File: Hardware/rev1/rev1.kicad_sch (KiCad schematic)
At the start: 0 parts

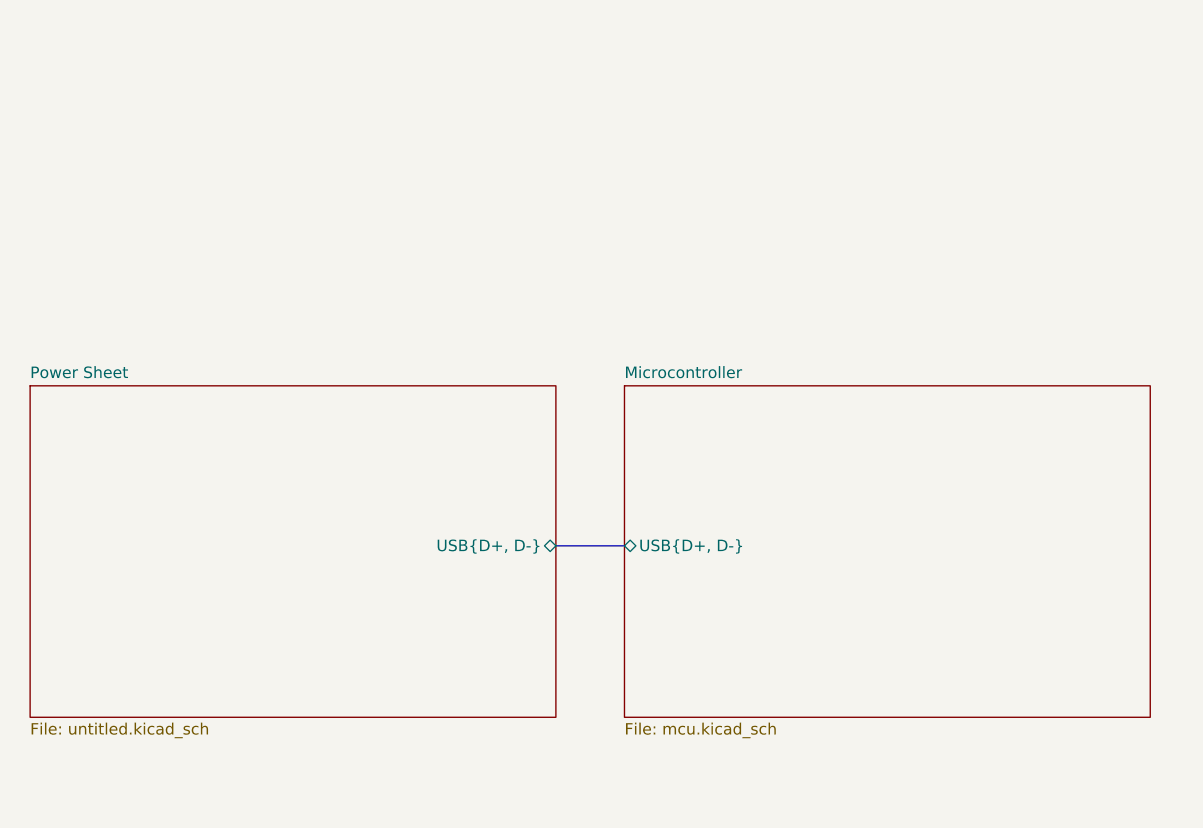
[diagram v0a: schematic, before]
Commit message: Add buses (maybe)
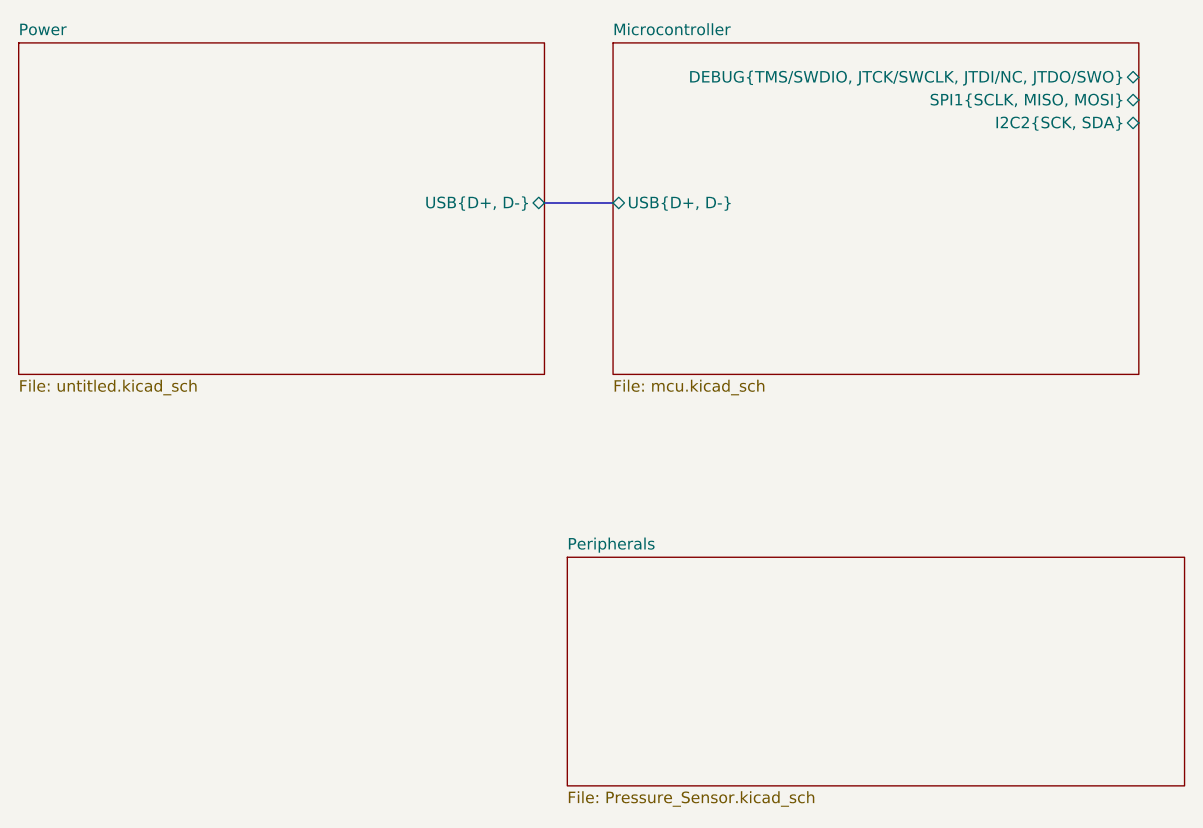
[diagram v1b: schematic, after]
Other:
- sheet Power Sheet renamed Power
- added sheet Peripherals (Pressure_Sensor.kicad_sch)
- sheet Microcontroller ports: added DEBUG{TMS/SWDIO, JTCK/SWCLK, JTDI/NC, JTDO/SWO}, I2C2{SCK, SDA}, SPI1{SCLK, MISO, MOSI}; removed none
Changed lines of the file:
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@@
 	(bus
 		(pts
-			(xy 144.78 95.25) (xy 152.4 95.25)
+			(xy 143.51 57.15) (xy 151.13 57.15)
 		)
 		(stroke
@@
 	)
 	(sheet
-		(at 152.4 77.47)
+		(at 151.13 39.37)
 		(size 58.42 36.83)
 		(fields_autoplaced yes)
@@
 		)
 		(property "Sheetname" "Microcontroller"
-			(at 152.4 76.7584 0)
+			(at 151.13 38.6584 0)
 			(effects
 				(font
@@
 		)
 		(property "Sheetfile" "mcu.kicad_sch"
-			(at 152.4 114.8846 0)
+			(at 151.13 76.7846 0)
 			(effects
 				(font
@@
 		)
 		(pin "USB{D+, D-}" bidirectional
-			(at 152.4 95.25 180)
+			(at 151.13 57.15 180)
 			(effects
 				(font
@@
 			)
 		)
+		(pin "DEBUG{TMS{slash}SWDIO, JTCK{slash}SWCLK, JTDI{slash}NC, JTDO{slash}SWO}"
+			bidirectional
+			(at 209.55 43.18 0
+			)
+			(effects
+				(font
+					(size 1.27 1.27)
+				)
+				(justify right)
+			)
+		)
+		(pin "SPI1{SCLK, MISO, MOSI}" bidirectional
+			(at 209.55 45.72 0)
+			(effects
+				(font
+					(size 1.27 1.27)
+				)
+				(justify right)
+			)
+		)
+		(pin "I2C2{SCK, SDA}" bidirectional
+			(at 209.55 48.26 0)
+			(effects
+				(font
+					(size 1.27 1.27)
+				)
+				(justify right)
+			)
+		)
 		(instances
 			(project "rev1"
 				(path "/e52639ab-1647-4d34-8bc5-5aadc4708147"
-					(page "5")
+					(page "3")
 				)
 			)
@@
 	)
 	(sheet
-		(at 86.36 77.47)
+		(at 85.09 39.37)
 		(size 58.42 36.83)
 		(fields_autoplaced yes)
@@
 			(color 0 0 0 0.0000)
 		)
-		(property "Sheetname" "Power Sheet"
-			(at 86.36 76.7584 0)
+		(property "Sheetname" "Power"
+			(at 85.09 38.6584 0)
 			(effects
 				(font
@@
 		)
 		(property "Sheetfile" "untitled.kicad_sch"
-			(at 86.36 114.8846 0)
+			(at 85.09 76.7846 0)
 			(effects
 				(font
@@
 		)
 		(pin "USB{D+, D-}" bidirectional
-			(at 144.78 95.25 0)
+			(at 143.51 57.15 0)
 			(effects
 				(font
@@
 				)
 			)
+		)
+	)
+	(sheet
+		(at 146.05 96.52)
+		(size 68.58 25.4)
+		(fields_autoplaced yes)
+		(stroke
+			(width 0.1524)
+			(type solid)
+		)
+		(fill
+			(color 0 0 0 0.0000)
+		)
+		(property "Sheetname" "Peripherals"
+			(at 146.05 95.8084 0)
+			(effects
+				(font
+					(size 1.27 1.27)
+				)
+				(justify left bottom)
+			)
+		)
+		(property "Sheetfile" "Pressure_Sensor.kicad_sch"
+			(at 146.05 122.5046 0)
+			(effects
+				(font
+					(size 1.27 1.27)
+				)
+				(justify left top)
+			)
+		)
+		(property "Field2" ""
+			(at 146.05 96.52 0)
+			(effects
+				(font
+					(size 1.27 1.27)
+				)
+				(hide yes)
+			)
+		)
+		(instances
+			(project "rev1"
+				(path "/e52639ab-1647-4d34-8bc5-5aadc4708147"
+					(page "4")
+				)
+			)
